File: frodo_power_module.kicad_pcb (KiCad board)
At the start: 2 copper layers, 56 x 71.2 mm, 78 parts, among them J1 Keystone 1098, J10 SWD Header, J2 Molex MicroFit 2x2, J3 Molex MicroFit 2x2, J4 Molex MicroFit 2x2, J5 Molex MicroFit 2x2, J6 Molex MicroFit 2x2, J7 JST-GH, J8 JST-GH, J9 JST-GH, U1 STM32F042F6Px, U2 L7805, U3 AZ1117I-3.3, U4 BQ25171-Q1, U5 BQ29200, U6 MCP2562-E-SN, U7 INA213, Y1 8MHz, 12p

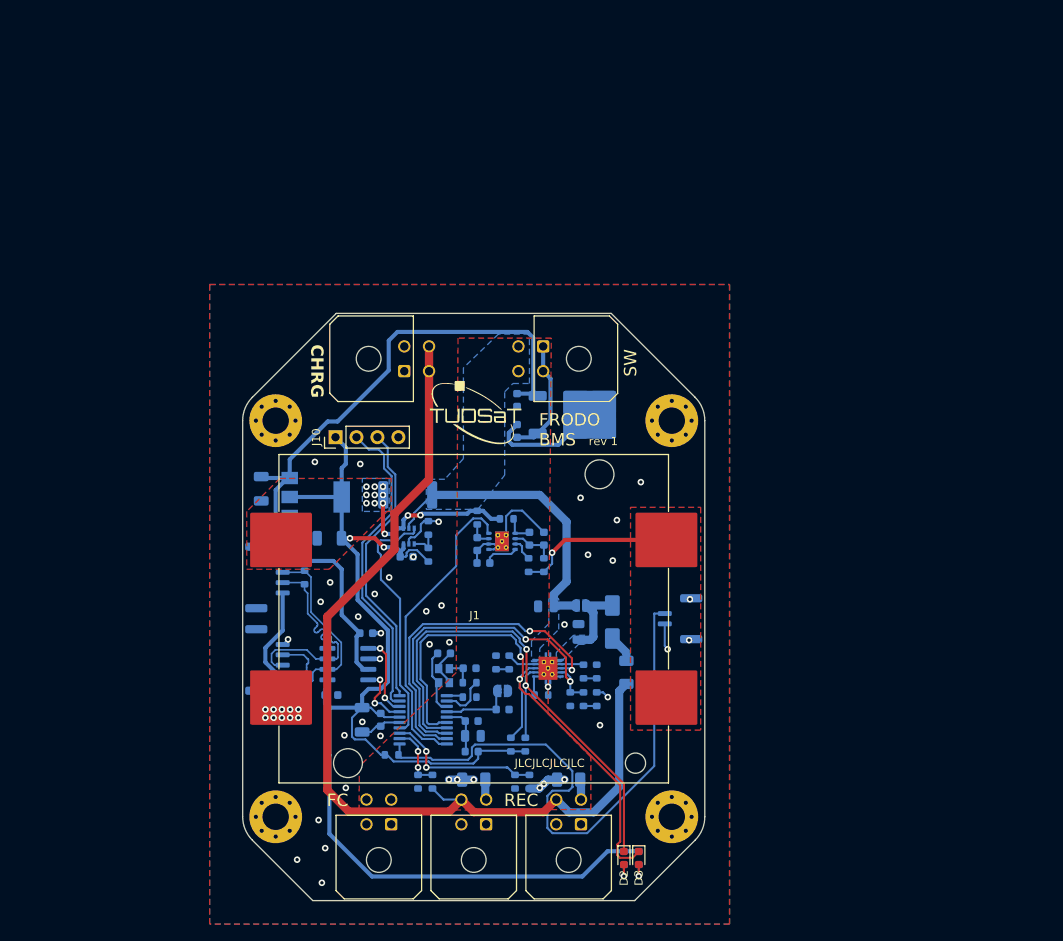
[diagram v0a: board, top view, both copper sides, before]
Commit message: worked on pcb
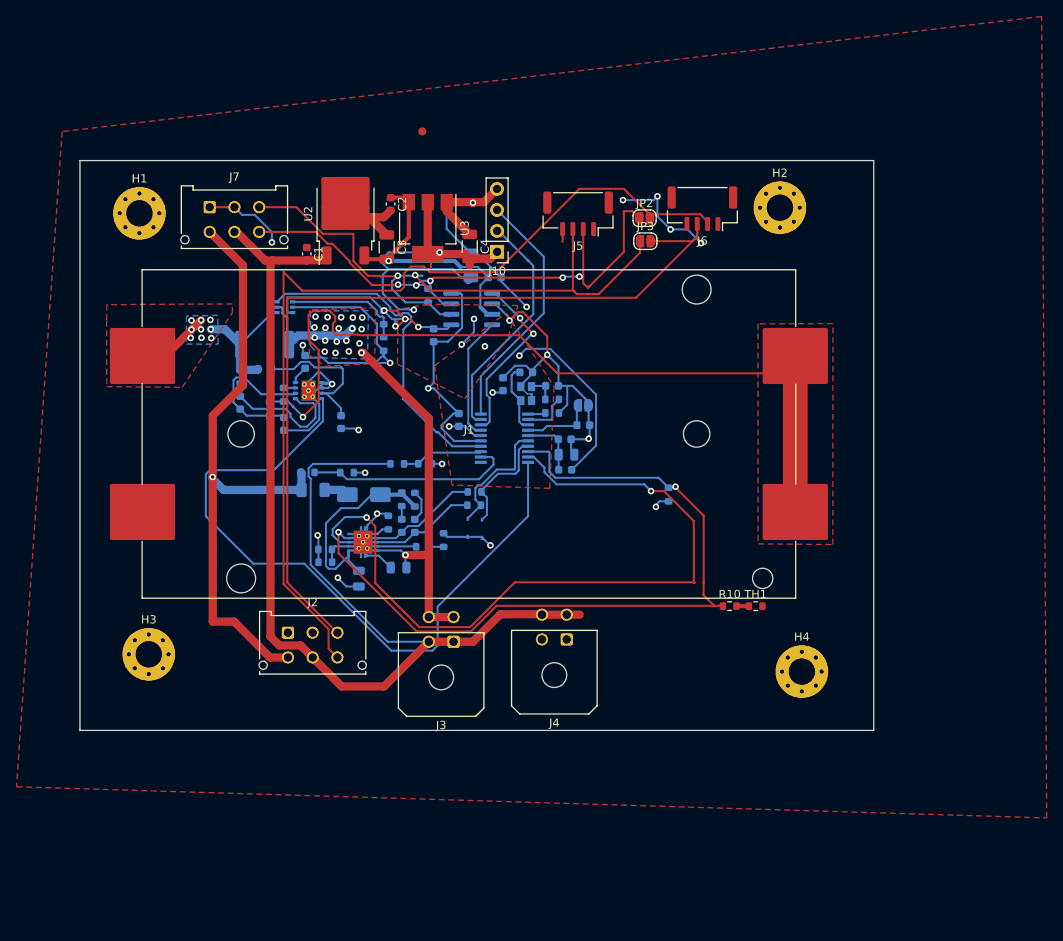
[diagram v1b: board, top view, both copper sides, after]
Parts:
- removed F2, F3: 1.5A, Fuse:Fuse_1206_3216Metric
- removed J8: JST-GH, Connector_JST:JST_GH_SM04B-GHS-TB_1x04-1MP_P1.25mm_Horizontal
- removed J9: JST-GH, Connector_JST:JST_GH_SM02B-GHS-TB_1x02-1MP_P1.25mm_Horizontal
- removed R11, R12, R2: 10k, Resistor_SMD:R_0603_1608Metric
- added D5: 3V9, footprints:SOD323F_DIO-L, B.Cu at (125.0, 113.1)
- added D6: 3V9, footprints:SOD323F_DIO-L, B.Cu at (123.3, 113.0)
- added JP3: SolderJumper_2_Open, Jumper:SolderJumper-2_P1.3mm_Open_RoundedPad1.0x1.5mm, F.Cu at (144.8, 78.3)
- added R27: 22k, Resistor_SMD:R_0603_1608Metric, B.Cu at (124.1, 108.6)
- added R28: 22k, Resistor_SMD:R_0603_1608Metric, B.Cu at (124.1, 110.2)
- C1, C2, C3, C4, JP2, R10, TH1, U2, U3: moved to F.Cu
- D2, D3: moved to B.Cu
- J1: value Keystone 1098 -> Keystone 1048; footprint frodo_power_module:keystone_1098 -> frodo_power_module:keystone_1048
- J2: value Molex MicroFit 2x2 -> Molex MicroFit 2x3; footprint Connector_Molex:Molex_Micro-Fit_3.0_43045-0400_2x02_P3.00mm_Horizontal -> Connector_Molex:Molex_Micro-Fit_3.0_43045-0612_2x03_P3.00mm_Vertical
- J5, J6: value Molex MicroFit 2x2 -> JST-GH; footprint Connector_Molex:Molex_Micro-Fit_3.0_43045-0400_2x02_P3.00mm_Horizontal -> Connector_JST:JST_GH_SM04B-GHS-TB_1x04-1MP_P1.25mm_Horizontal
- J7: value JST-GH -> Molex MicroFit 2x3; footprint Connector_JST:JST_GH_SM04B-GHS-TB_1x04-1MP_P1.25mm_Horizontal -> Connector_Molex:Molex_Micro-Fit_3.0_43045-0612_2x03_P3.00mm_Vertical; moved to F.Cu
- R25, R26: value 1k -> 1k5
- R7: value 220 -> 1k
- R8: value 220 -> 680
- moved J6 76.0 mm to (151.7, 74.3)
- moved J5 74.8 mm to (136.6, 74.9)
- moved JP2 59.8 mm to (144.7, 75.5)
- moved C5 56.6 mm to (123.7, 81.2), turned to -90 degrees
- moved R26 51.2 mm to (116.9, 109.6), turned to 90 degrees
- moved R25 51.1 mm to (115.3, 109.5)
- moved D3 48.5 mm to (116.9, 112.7), turned to 90 degrees
- moved D2 48.4 mm to (115.3, 112.7), turned to 90 degrees
- moved C19 45.8 mm to (126.5, 82.6)
- moved U6 45.6 mm to (123.8, 86.5)
- moved J7 45.4 mm to (92.0, 74.1), turned to 0 degrees
- moved F1 43.9 mm to (104.5, 108.4), turned to 0 degrees
- moved C6 43.3 mm to (127.6, 95.6), turned to -90 degrees
- moved R22 41.7 mm to (114.7, 105.2), turned to 0 degrees
- moved R20 40.4 mm to (103.9, 106.3), turned to 0 degrees
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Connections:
- D2 pad 1: STAT1 -> Net-(D2-K)
- D3 pad 1: STAT2 -> Net-(D3-K)
- J2 pad 3: VDC -> Net-(J2-Pin_3)
- J5 pad 1: GND -> unconnected-(J5-Pin_1-Pad1)
- J5 pad 2: GND -> CAN+
- J5 pad 3: Net-(J5-Pin_3) -> CAN-
- J5 pad 4: VDC -> GND
- J6 pad 1: GND -> unconnected-(J6-Pin_1-Pad1)
- J6 pad 2: GND -> Net-(J2-Pin_6)
- J6 pad 3: Net-(J6-Pin_3) -> Net-(J2-Pin_3)
- J6 pad 4: VDC -> GND
- J7 pad 1: Net-(J7-Pin_1) -> GND
- J7 pad 2: CAN+ -> GND
- J7 pad 4: GND -> VDC
- JP1 pad 1: Net-(D1-K) -> NRST
- JP1 pad 2: +BATT -> GND
- JP2 pad 1: NRST -> CAN+
- JP2 pad 2: GND -> Net-(J2-Pin_6)
- R25 pad 1: +3V3 -> Net-(D1-K)
- R26 pad 1: +3V3 -> Net-(D1-K)
- R7 pad 2: Net-(R7-Pad2) -> GND
- R8 pad 1: Net-(R7-Pad2) -> Net-(U4-ISET)
- U1 pad 11: BREAKWIRE -> unconnected-(U1-PA5-Pad11)
- U4 pad 7: STAT1 -> Net-(D2-K)
- U4 pad 8: STAT2 -> Net-(D3-K)
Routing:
- net GND: track 52.9 -> 227.3 mm, vias 46 -> 22
- net +VSW: track 22.0 -> 142.3 mm, vias 6 -> 0
- net Net-(J2-Pin_6): track 0.00 -> 110.9 mm
- net Net-(J2-Pin_3): track 0.00 -> 104.8 mm
- net Net-(J1-Pin_2): track 19.1 -> 102.3 mm
- net BREAKWIRE: track 71.1 -> 0.00 mm
- net STAT2: track 69.9 -> 15.1 mm, vias 2 -> 0
- net STAT1: track 66.4 -> 13.4 mm, vias 2 -> 0
- net +5V: track 85.1 -> 32.9 mm, vias 0 -> 1
- net NTC: track 43.1 -> 93.3 mm
- net CHARGE_ENABLE: track 40.5 -> 90.6 mm
- net BLNCR_OUT: track 37.3 -> 86.5 mm
- net CAN-: track 27.8 -> 75.6 mm, vias 0 -> 2
- net +3V3: track 155.4 -> 108.3 mm, vias 2 -> 12
- net CAN+: track 27.7 -> 71.9 mm, vias 0 -> 5
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- added copper zone on F.Cu, net +3V3
- added copper zone on F.Cu, net +BATT
- removed copper zone on F.Cu, net +VSW
- removed copper zone on B.Cu, net GND
- removed copper zone on B.Cu, net Net-(D1-K)
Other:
- board size 56 x 71.2 mm -> 96.2 x 69 mm
- board text removed: "FRODO BMS"
- board text removed: "JLCJLCJLCJLC"
- board text removed: "rev 1"
